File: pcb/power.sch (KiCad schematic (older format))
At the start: 17 parts

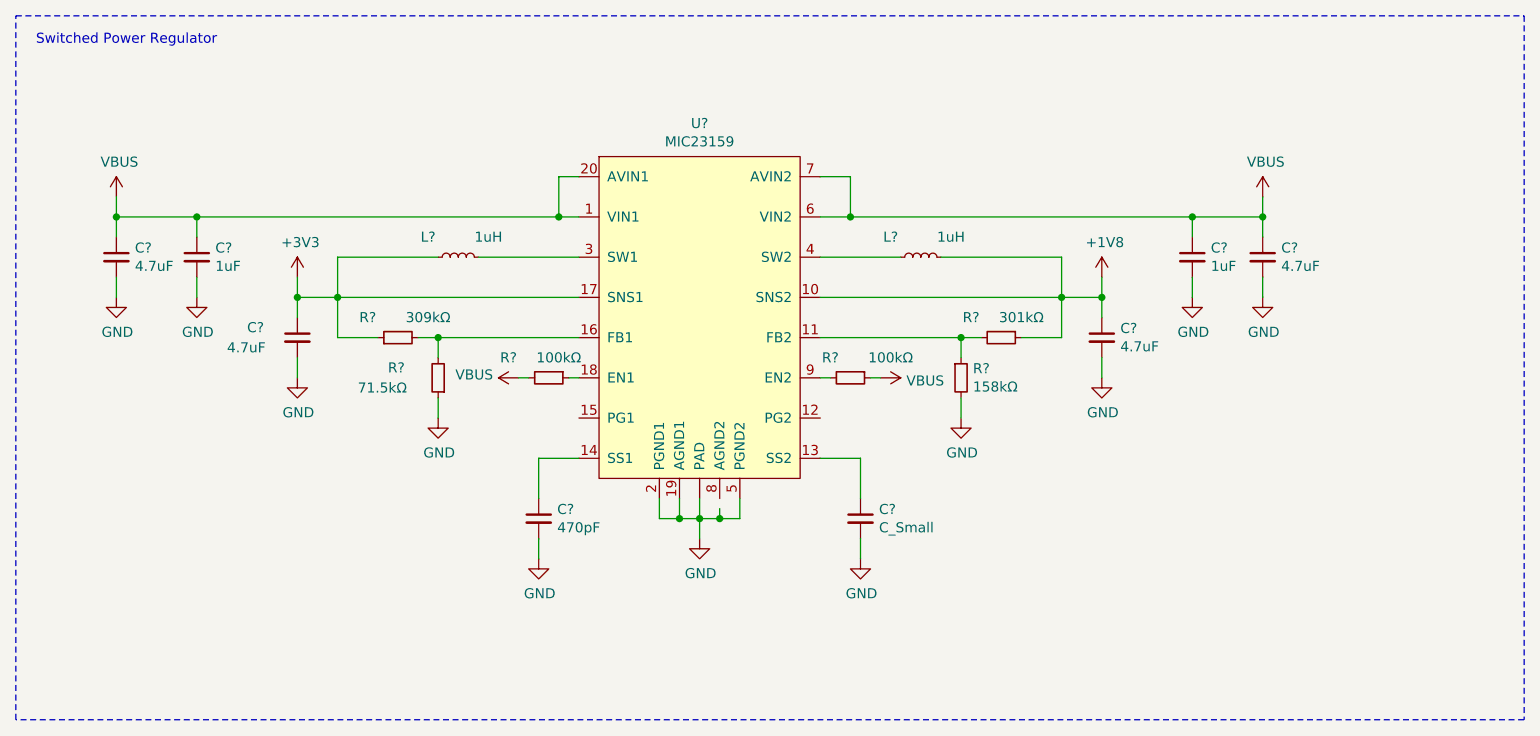
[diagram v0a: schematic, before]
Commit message: SCH: minor changes
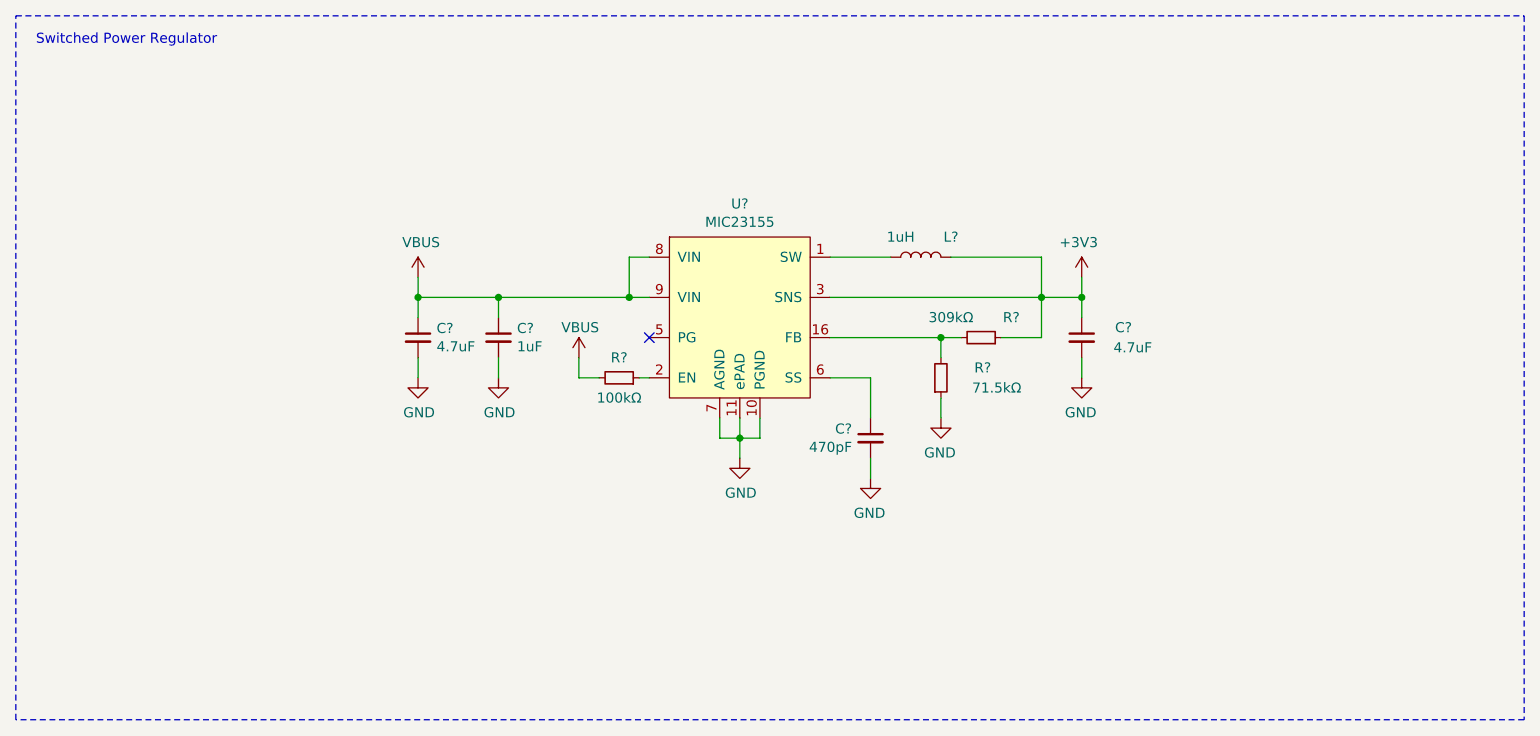
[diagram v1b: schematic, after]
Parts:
- removed C?: 1uF, symbol Device:C_Small
- removed C? (x2): 4.7uF, symbol Device:C_Small
- removed C?: C_Small, symbol Device:C_Small
- removed L? (x2): 1uH, symbol Device:L_Small
- removed R?: 100kΩ, symbol Device:R_Small
- removed R?: 158kΩ, symbol Device:R_Small
- removed R?: 301kΩ, symbol Device:R_Small
- removed U?: MIC23159, symbol rs_Regulator_switching:MIC23159
- added L?: 1uH, symbol Device:L
- added U?: MIC23155, symbol rs_Regulator_switching:MIC23155
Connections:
- net +3V3: now also L?.1, U?.3 (SNS)
- net GND: now also U?.10 (PGND), U?.11 (ePAD), U?.7 (AGND)
- net VBUS: now also U?.8 (VIN), U?.9 (VIN)
- net at C?.1: now also U?.6 (SS)
- net at R?.2, R?.2: now also U?.16 (FB)
- net at R?.1: now also U?.2 (EN)
- new net: L?.2, U?.1 (SW)
- no-connect marks 0 -> 1
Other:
- moved on the sheet: C?, R?
